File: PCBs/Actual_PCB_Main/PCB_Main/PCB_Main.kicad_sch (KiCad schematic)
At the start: 135 parts, among them J1 LED Connectors+, J10 To_Speaker_R, J2 fan connector, J3 USB_B_Micro, J4 USB_B_Micro, J5 LED connectors -, J6 XT60-M, J7 HUB75, J9 To_Speaker_L, M1 CSD17581Q3, M2 CSD17581Q3A, Q1 S8050, Q2 S8050, Q3 NMOS, Q5 S8050, Q6 S8050, SW1 SW_Push, SW2 SW_Push, SW3 SW_Push, SW4 SW_Push, U1 CP2102N-Axx-xQFN28, U2 AMS1117-3.3, U3 ESP32-WROOM-E, U4 PCM5102A, U5 LM5122MH/NOPB, U6 ESP32-WROVER-E, U7 LM4752TS, U9 CP2102N-Axx-xQFN28, Y1 CB3LV-3I-40M000000, Y2 CB3LV-3I-40M000000

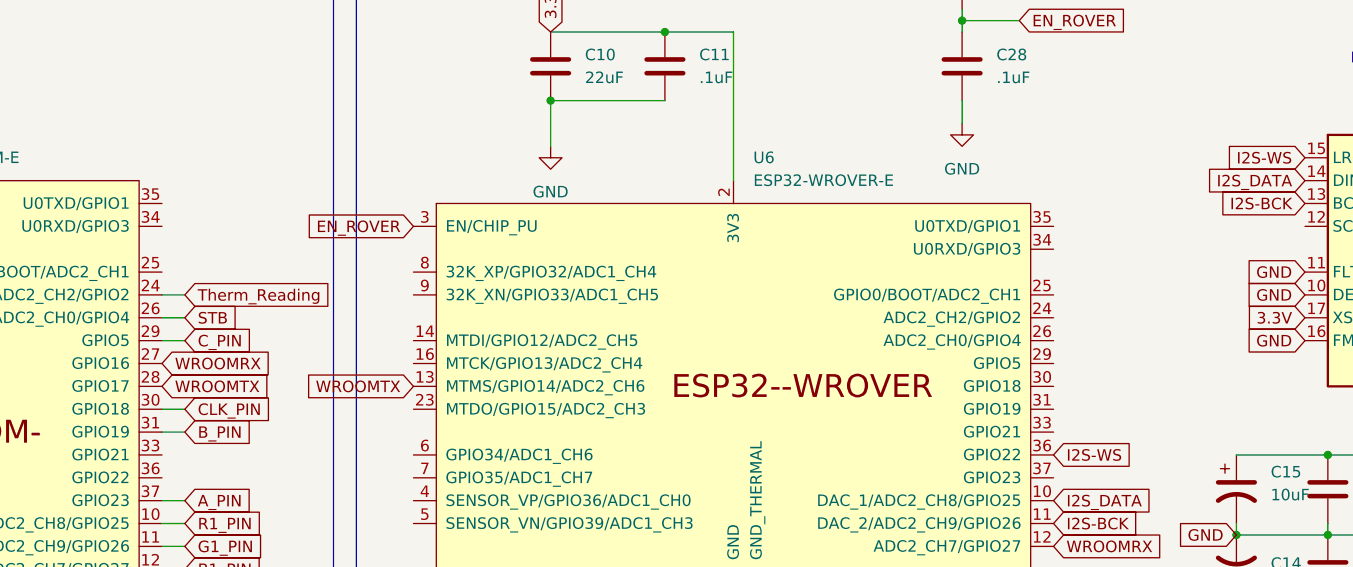
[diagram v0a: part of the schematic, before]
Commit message: BOOT
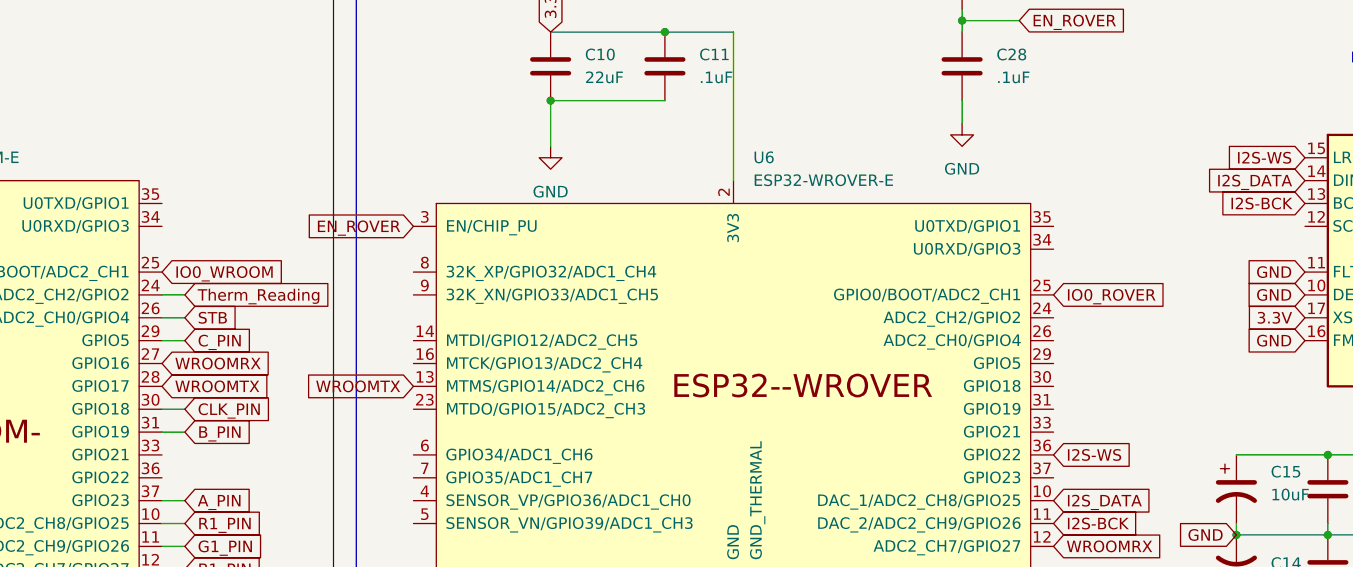
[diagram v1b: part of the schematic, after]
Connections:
- net IO0_ROVER: now also U6.25 (GPIO0/BOOT/ADC2_CH1)
- net IO0_WROOM: now also U3.25 (GPIO0/BOOT/ADC2_CH1)
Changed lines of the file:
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@@
+    )
+  )
+  (global_label "IO0_ROVER" (shape input) (at 194.31 99.06 0) (fields_autoplaced)
+    (effects (font (size 1.27 1.27)) (justify left))
+    (property "Intersheetrefs" "${INTERSHEET_REFS}" (at 207.5157 99.06 0)
+      (effects (font (size 1.27 1.27)) (justify left) hide)
     )
   )
@@
       (effects (font (size 1.27 1.27)) (justify left) hide)
     )
+  )
+  (global_label "IO0_WROOM" (shape input) (at 95.25 96.52 0) (fields_autoplaced)
+    (effects (font (size 1.27 1.27)) (justify left))
+    (property "Intersheetrefs" "${INTERSHEET_REFS}" (at 109.1814 96.52 0)
+      (effects (font (size 1.27 1.27)) (justify left) hide)
+    )

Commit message: finished schematic
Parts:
- removed D10, D11, D12, D13, D2, D3, D4, D5: BZX84Cxx, Package_TO_SOT_SMD:SOT-23, symbol Diode:BZX84Cxx
- removed D6: RED LED, LED_SMD:LED_0805_2012Metric, symbol Device:LED
- removed J1: LED Connectors+, symbol Connector:Conn_01x03_Pin
- removed J2: fan connector, symbol Connector:Conn_01x02_Pin
- removed J3, J4: USB_B_Micro, symbol Connector:USB_B_Micro
- removed J5: LED connectors -, symbol Connector:Conn_01x03_Pin
- removed Q3: NMOS, symbol Simulation_SPICE:NMOS
- added Boot2ROVER1, Boot2WROOM1: ~, Artisyn_Components:USB_TO_TTL_FT232RL, symbol Interface:USB_TO_TTL_FT232RL
- added C30: 10uF, Capacitor_SMD:C_0805_2012Metric, symbol Device:C
- added C34, CsnR2, CsnR3: .1uF, Capacitor_SMD:C_0805_2012Metric, symbol Device:C
- added D10, D11, D12, D13, D14, D6, D8, D9: MM5Zxx, Diode_SMD:D_SOD-523, symbol Diode:MM5Zxx
- added D7: RED LED, LED_SMD:LED_0805_2012Metric, symbol Device:LED
- added H1, H2, H3, H4: MountingHole, MountingHole:MountingHole_2.7mm, symbol Mechanical:MountingHole
- added J1: fan connector, Connector_PinHeader_2.54mm:PinHeader_1x02_P2.54mm_Vertical, symbol Connector:Conn_01x02_Pin
- added J2, J4: 10118193-0001LF, Artisyn_Components:Artysin_USB_CONN, symbol Artysin_USB_CONN:10118193-0001LF
- added Q4: Fan_NMOS, Artisyn_Components:Fan_MOSFET, symbol Fan_MOSFET:SI1902CDL-T1-BE3
- added R20: 1k, Resistor_SMD:R_0815_2038Metric, symbol Device:R
- added R21: 500, Resistor_SMD:R_0805_2012Metric, symbol Device:R
- C1: value 22uF -> 10uF
- C2: value 22uF -> .1uF
- C25, C26, C27, C29: footprint (none) -> Capacitor_SMD:C_0805_2012Metric
- R19: value 1k -> 500; footprint (none) -> Resistor_SMD:R_0805_2012Metric
- Y1, Y2: footprint CB3LV-3I-40M000000:OSC_CB3LV-3I-40M000000 -> Artisyn_Components:Onboard_Clock
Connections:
- net 3.3V: now also Boot2ROVER1.4 (VCC), Boot2WROOM1.4 (VCC), C30.1, CsnR2.1, CsnR3.1
- net GND: now also Csc1.2, Boot2ROVER1.6 (GND), Boot2WROOM1.6 (GND), C30.2, C34.2, CsnR2.2, CsnR3.2, D11.2 (A), D12.2 (A), D13.2 (A), D6.2 (A), D8.2 (A), D9.2 (A), J2.5 (GND), J4.5 (GND), R20.2; no longer R19.2
- net RXD_ROVER: now also U6.34 (U0RXD/GPIO3), Boot2ROVER1.2 (RX)
- net RXD_WROOM: now also U3.35 (U0TXD/GPIO1), Boot2WROOM1.2 (RX)
- net TXD_ROVER: now also U6.35 (U0TXD/GPIO1), Boot2ROVER1.3 (TX)
- net TXD_WROOM: now also U3.34 (U0RXD/GPIO3), Boot2WROOM1.3 (TX)
- net USB_DN_ROVER: now also D8.1 (K)
- net USB_DN_WROOM: now also D12.1 (K)
- net USB_DP_ROVER: now also D9.1 (K)
- net USB_DP_WROOM: now also D13.1 (K)
- net VBUS_ROVER: now also D14.2 (A), D6.1 (K)
- net VBUS_WROOM: now also D10.2 (A), D11.1 (K)
- net VCC: now also C34.1, D10.1 (K), D14.1 (K), J1.2 (Pin_2)
- net WROOM_TO_FANS: now also U3.7 (GPIO35/ADC1_CH7), Q4.5 (G2)
- net at Cout1.1, Coutx1.1, Csc1.1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: now also C3b1.1
- net at R33.1: now also J4.2 (D-)
- net WROOM_TALK_RX: now reaches R19.1
- net WROOM_TALK_RX: now also U3.27 (GPIO16)
- net at R34.1: now also J4.3 (D+)
- net at R32.1: now also J4.1 (VUSB)
- net at R11.1: now also J2.2 (D-)
- net at R14.1: now also J2.1 (VUSB)
- net at R12.1: now also J2.3 (D+)
- net WROOMRX renamed ROVER_TALK_TX
- net ROVER_TALK_TX: now also R19.2; no longer U3.27 (GPIO16)
- net WROOMTX renamed ROVER_TALK_RX
- net ROVER_TALK_RX: now also R21.2; no longer U3.28 (GPIO17)
- new net: J1.1 (Pin_1), Q4.3 (D2)
- new net: D7.2 (A), Q4.4 (S2)
- new net: D7.1 (K), R20.1
- new net WROOM_TALK_TX: R21.1, U3.28 (GPIO17)
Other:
- note removed: "LED CONNECTORS"
- moved on the sheet: C10, C11, C12, C13, C14, C15, C16, C17, C18, C19, C2, C20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
